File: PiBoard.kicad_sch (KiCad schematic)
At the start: 4 parts

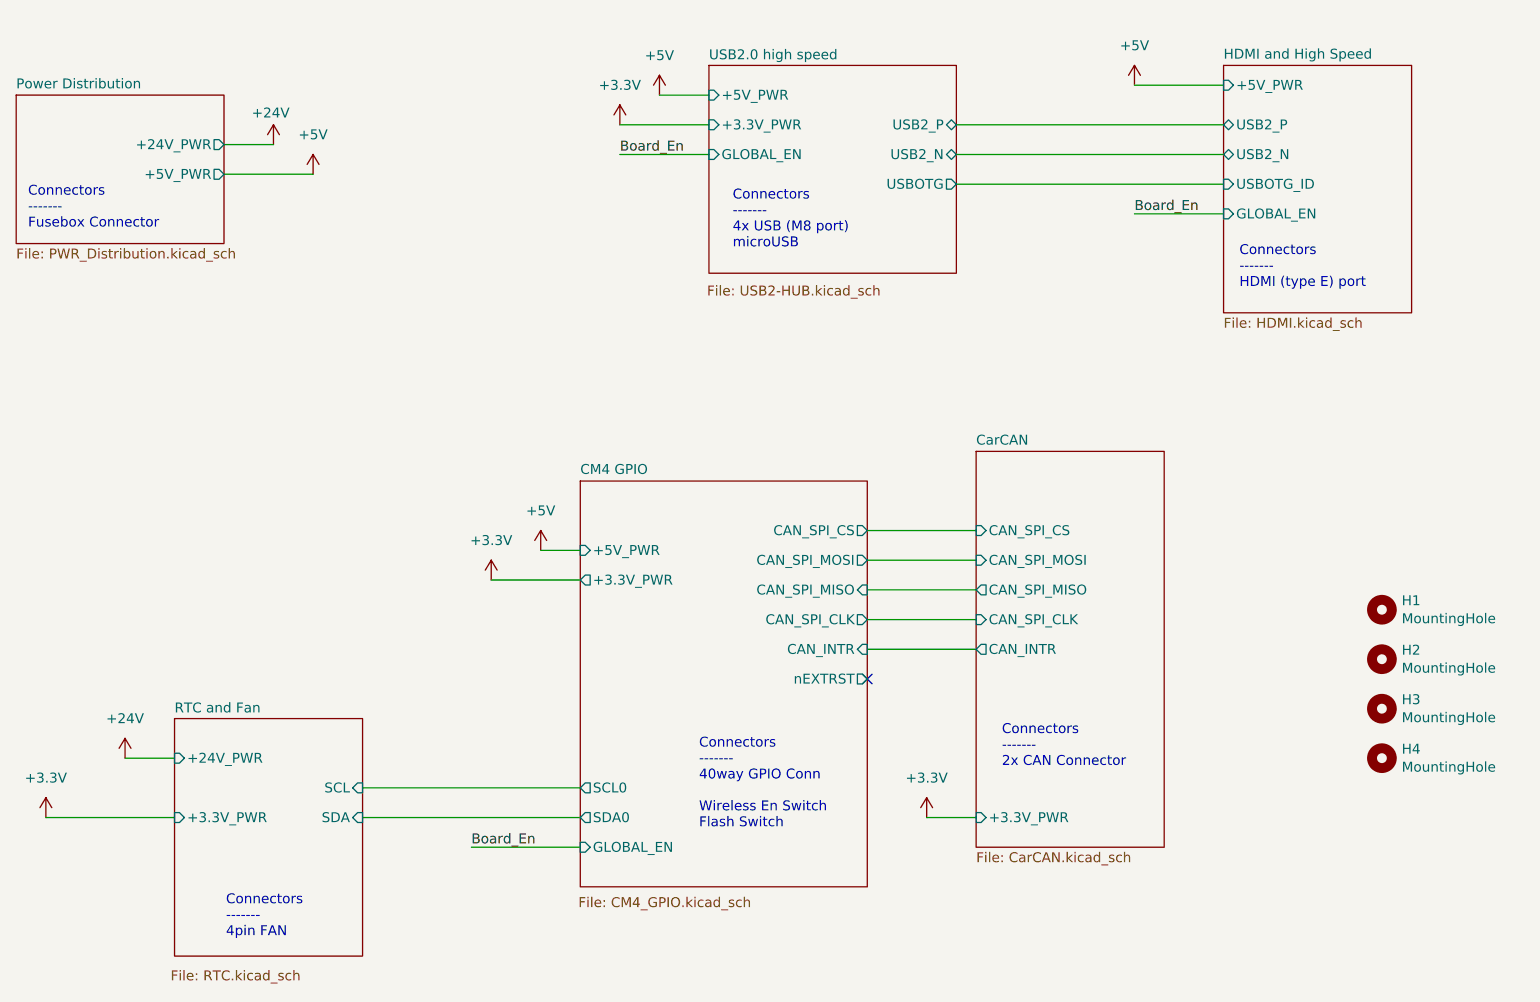
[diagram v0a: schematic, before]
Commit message: my life is horrible
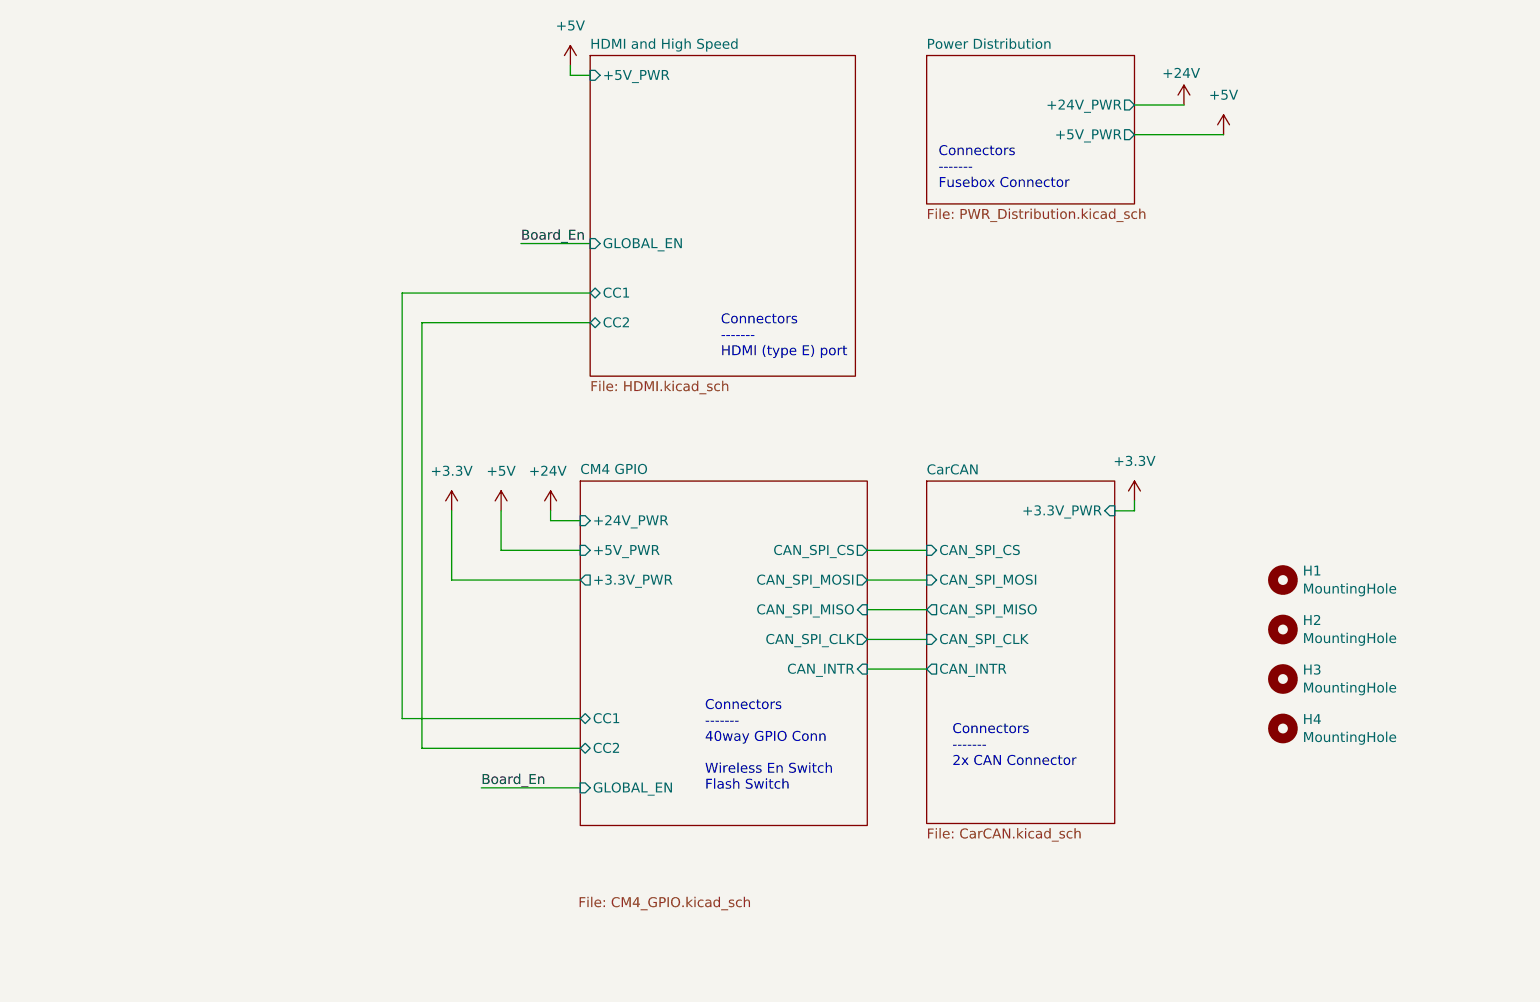
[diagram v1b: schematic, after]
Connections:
- no-connect marks 1 -> 0
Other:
- removed sheet RTC and Fan
- removed sheet USB2.0 high speed
- sheet CM4 GPIO ports: added +24V_PWR, CC1, CC2; removed SCL0, SDA0, nEXTRST
- sheet HDMI and High Speed ports: added CC1, CC2; removed USB2_N, USB2_P, USBOTG_ID
- note removed: "Connectors ------- 4pin FAN"
- note removed: "Connectors ------- 4x USB (M8 port) microUSB"
- moved on the sheet: H1, H2, H3, H4
